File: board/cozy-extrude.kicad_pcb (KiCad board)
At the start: 2 copper layers, 43.2 x 69.9 mm, 11 parts, among them J1 RPi-Pico-Socket, J2 BME280, J3 PWM-Fan, J4 Heater-Switch, K1 HF46F_5-HS1, U1 ULN2003

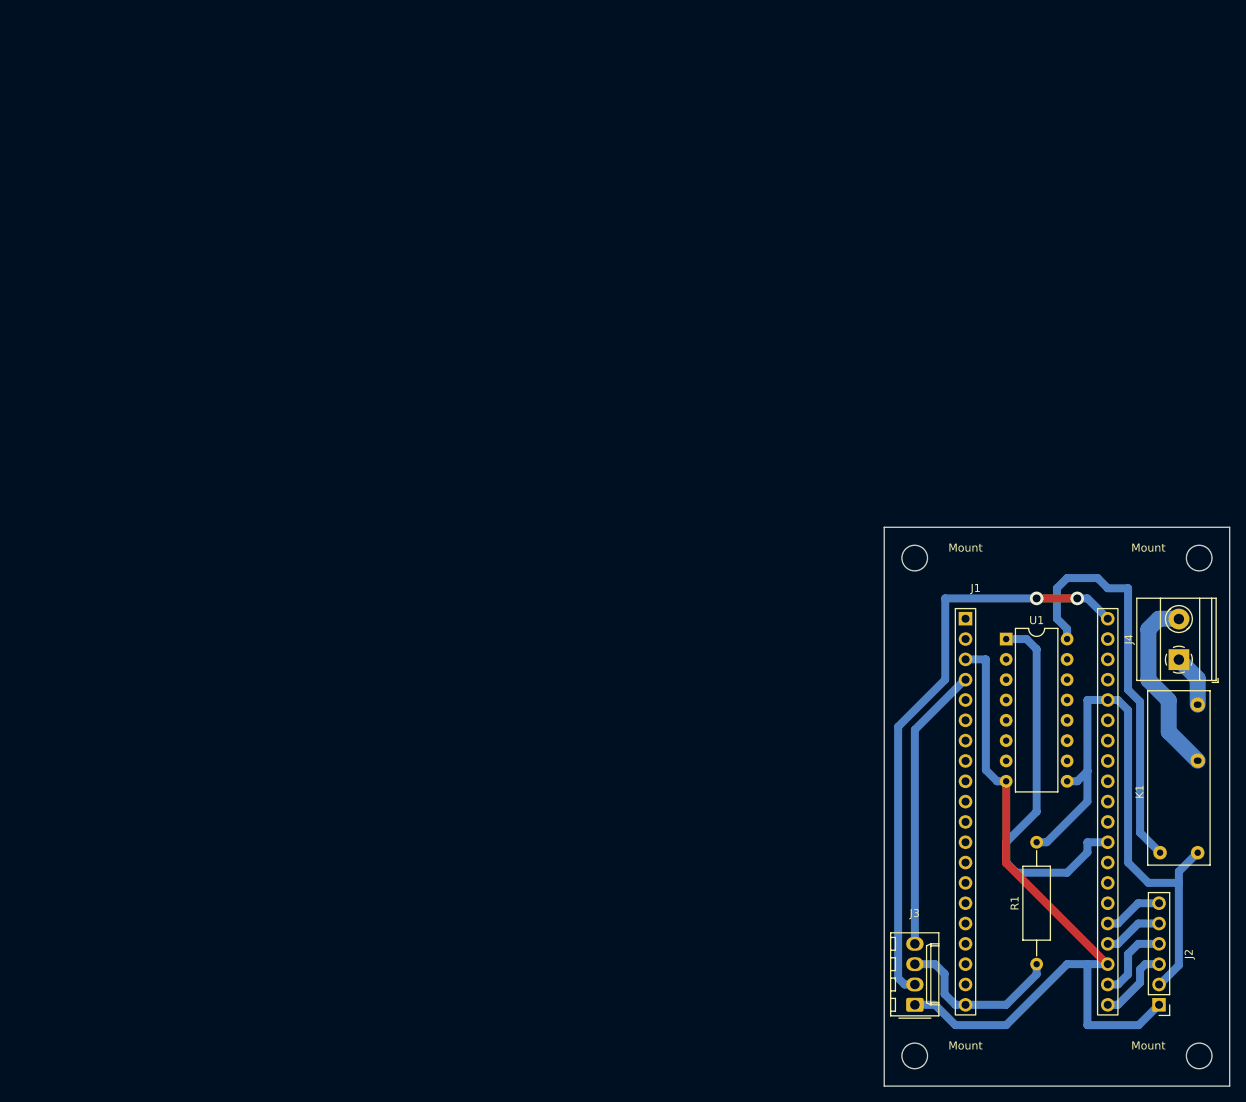
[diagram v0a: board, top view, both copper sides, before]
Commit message: improved pcb
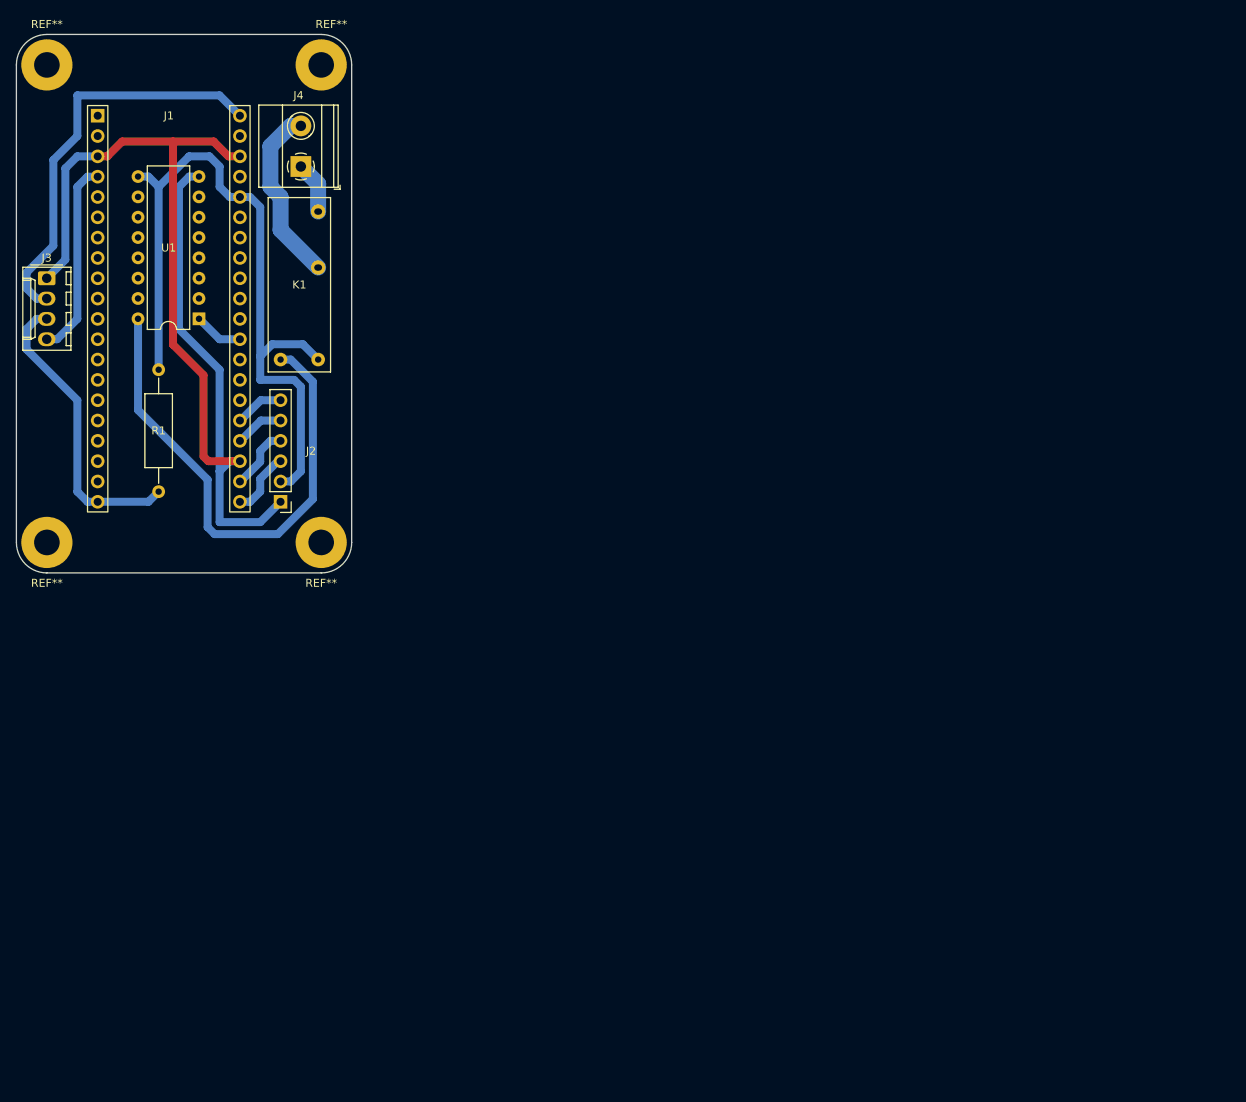
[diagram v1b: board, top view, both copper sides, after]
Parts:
- removed Mount (x4): MountingHole_3.2mm_M3, MountingHole:MountingHole_3.2mm_M3
- added REF**: MountingHole_3.2mm_M3_Pad, MountingHole:MountingHole_3.2mm_M3_Pad, F.Cu at (4.55, 64.1)
- added REF**: MountingHole_3.2mm_M3_Pad, MountingHole:MountingHole_3.2mm_M3_Pad, F.Cu at (4.55, 4.40)
- added REF**: MountingHole_3.2mm_M3_Pad, MountingHole:MountingHole_3.2mm_M3_Pad, F.Cu at (38.8, 4.40)
- added REF**: MountingHole_3.2mm_M3_Pad, MountingHole:MountingHole_3.2mm_M3_Pad, F.Cu at (38.8, 64.1)
- J2: value BME280 -> BME280 Conn
- J3: value PWM-Fan -> PWM Fan Conn
- R1: value TACH-Pullup -> 2.2k
- moved J3 141.5 mm to (4.53, 31.1), turned to -90 degrees
- moved J2 126.5 mm to (33.8, 59.0)
- moved K1 126.0 mm to (33.8, 41.2)
- moved J4 125.9 mm to (36.3, 17.1)
- moved J1 125.4 mm to (10.9, 10.7)
- moved R1 124.6 mm to (18.5, 57.7)
- moved U1 108.5 mm to (23.6, 36.1), turned to 180 degrees
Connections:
- J1 pad 38: unconnected-(J1-Pad38) -> GND
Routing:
- net GND: track 93.6 -> 143.2 mm
- net /HEATER_EN: track 48.1 -> 6.17 mm
- net VBUS: track 73.7 -> 51.2 mm, vias 2 -> 0
- net +3V3: track 74.8 -> 93.7 mm
- net /TACH: track 21.7 -> 37.2 mm
- net Net-(K1-Pad1): track 51.5 -> 64.8 mm
- net /PWM: track 35.7 -> 24.5 mm
- net /CSB: track 10.0 -> 7.97 mm
- net /SDO: track 9.49 -> 8.13 mm
- net /SCL: track 7.46 -> 6.13 mm
- net /SDA: track 7.46 -> 6.13 mm
- net Net-(K1-Pad3): track 23.7 -> 22.5 mm
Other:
- board size 43.2 x 69.9 mm -> 41.9 x 67.3 mm
